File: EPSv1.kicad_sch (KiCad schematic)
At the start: 0 parts

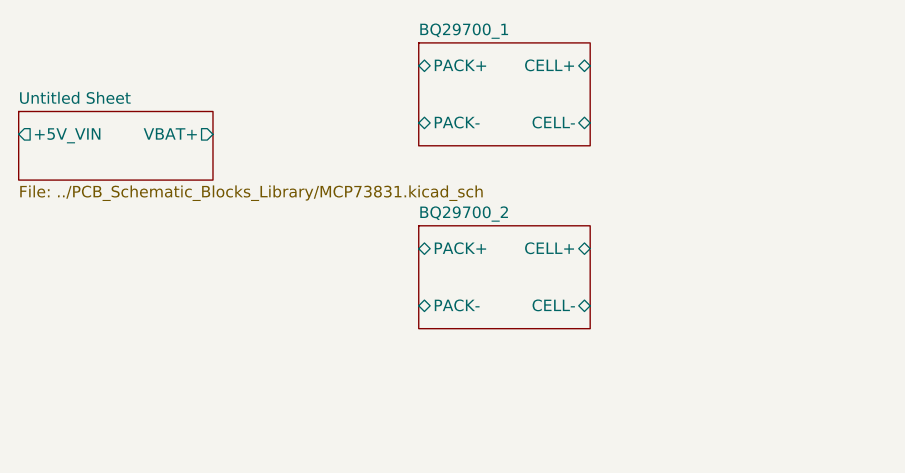
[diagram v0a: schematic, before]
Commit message: first commit
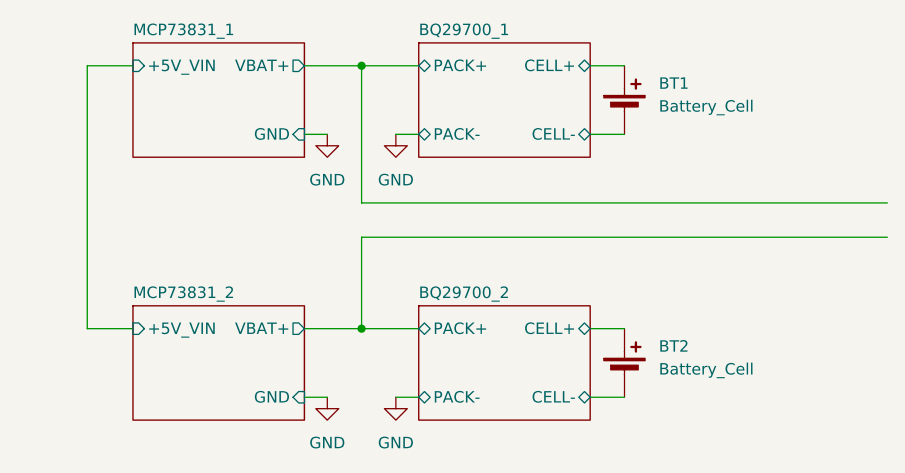
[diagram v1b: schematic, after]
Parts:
- added BT1, BT2: Battery_Cell, symbol Device:Battery_Cell
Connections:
- net BQ29700_1/CELL+: now also BT1.1 (+)
- net BQ29700_1/CELL-: now also BT1.2 (-)
- net BQ29700_2/CELL+: now also BT2.1 (+)
- net BQ29700_2/CELL-: now also BT2.2 (-)
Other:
- sheet Untitled Sheet renamed MCP73831_1
- added sheet MCP73831_2 (../PCB_Schematic_Blocks_Library/MCP73831.kicad_sch)
- sheet MCP73831_1 ports: added GND; removed none
